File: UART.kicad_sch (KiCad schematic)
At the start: 9 parts, among them U6 CP2102N-A02-GQFN28

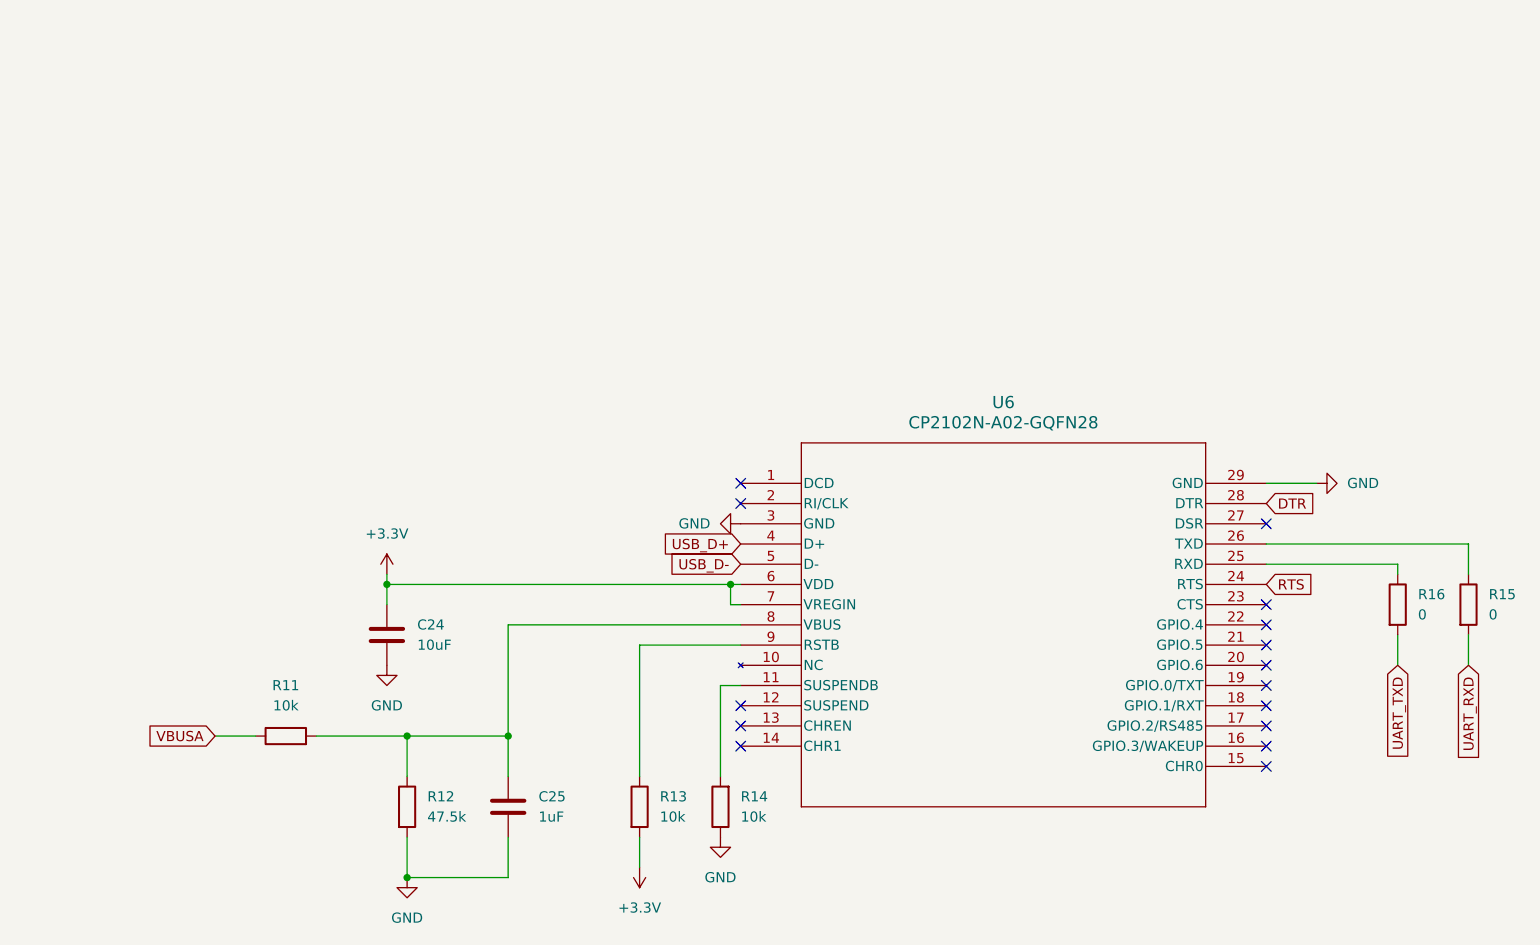
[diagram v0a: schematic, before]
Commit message: Moved some components around
No reason, just wanted to push to avoid merge conflicts
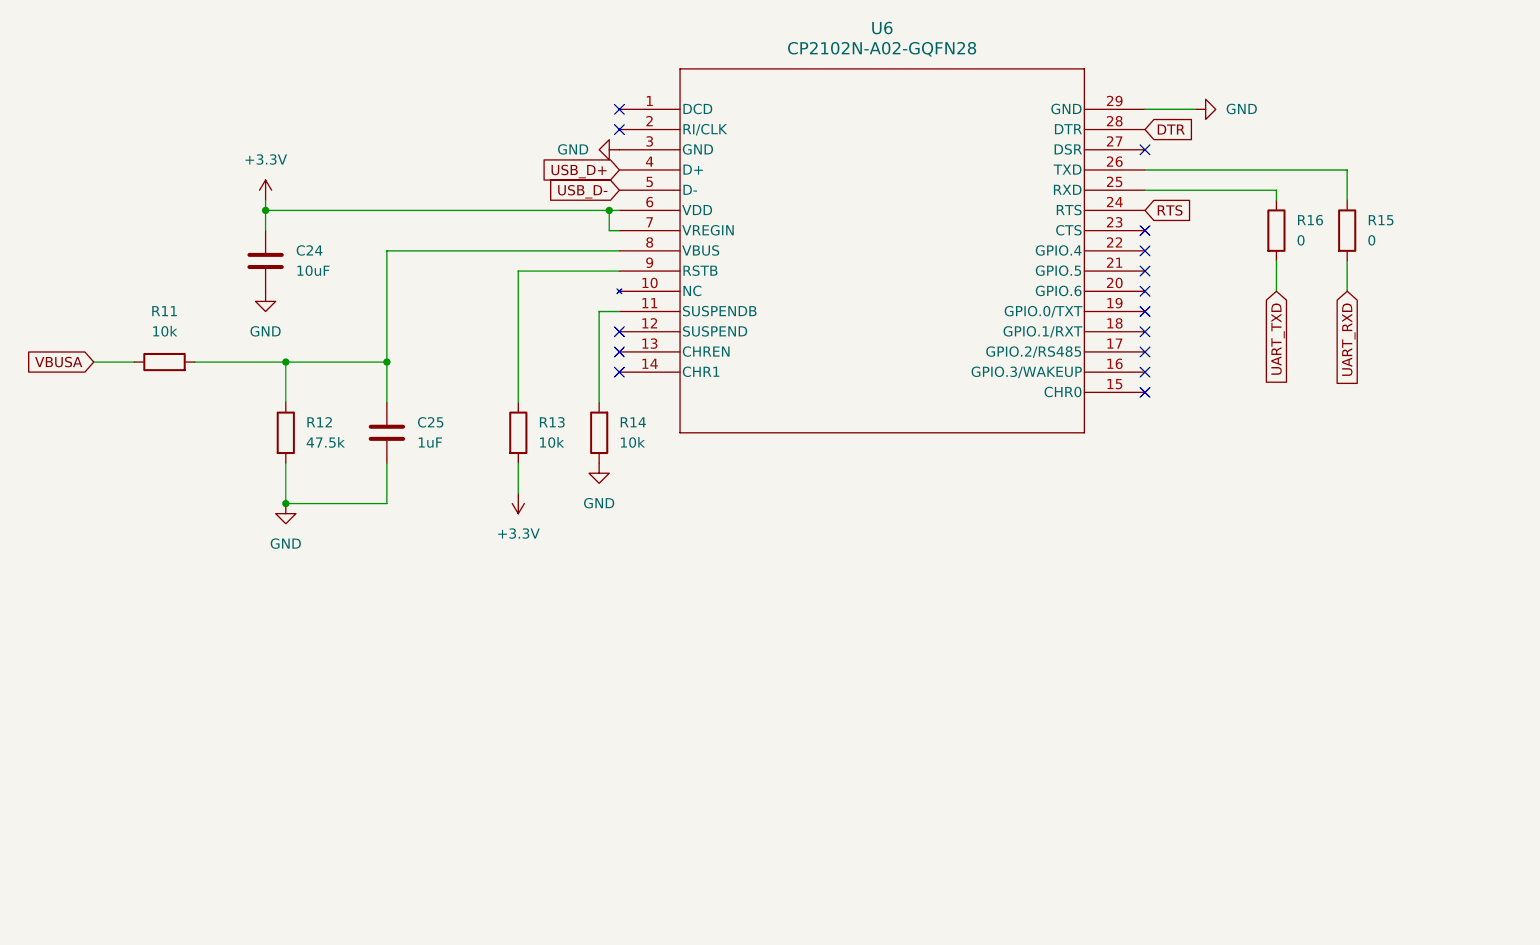
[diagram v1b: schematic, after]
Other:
- moved on the sheet: C24, C25, R11, R12, R13, R14, R15, R16, U6
